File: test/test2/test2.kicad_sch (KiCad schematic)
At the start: 2 parts, among them U1 module_mpu6050, U2 mini_esp32

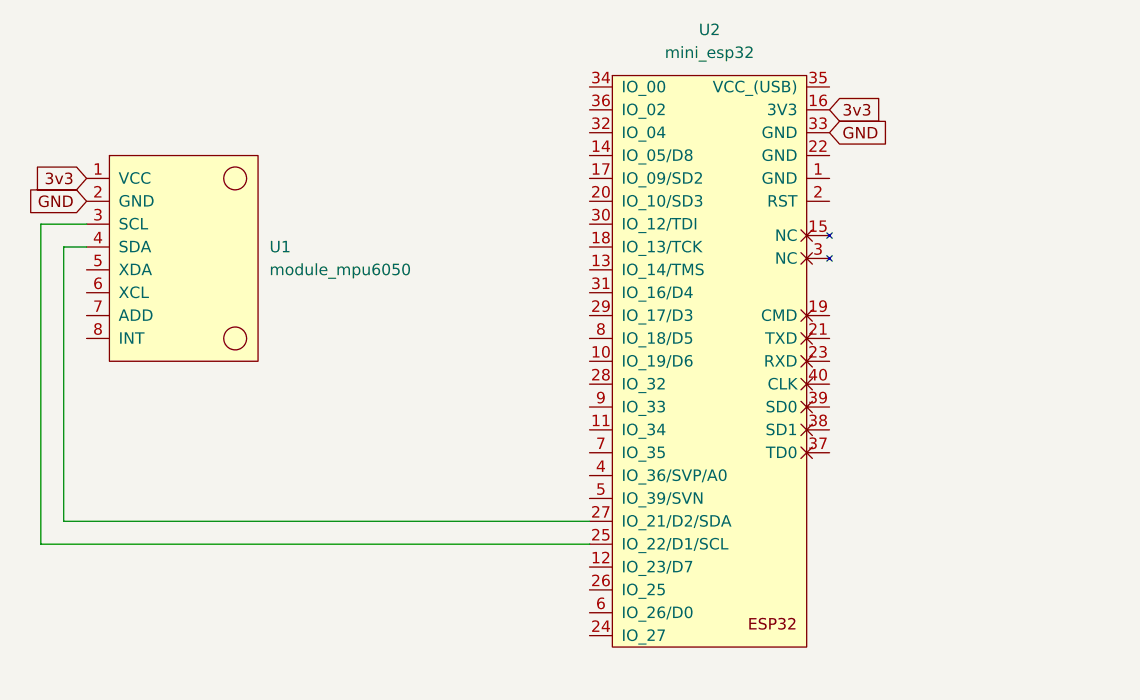
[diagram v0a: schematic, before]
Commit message: update
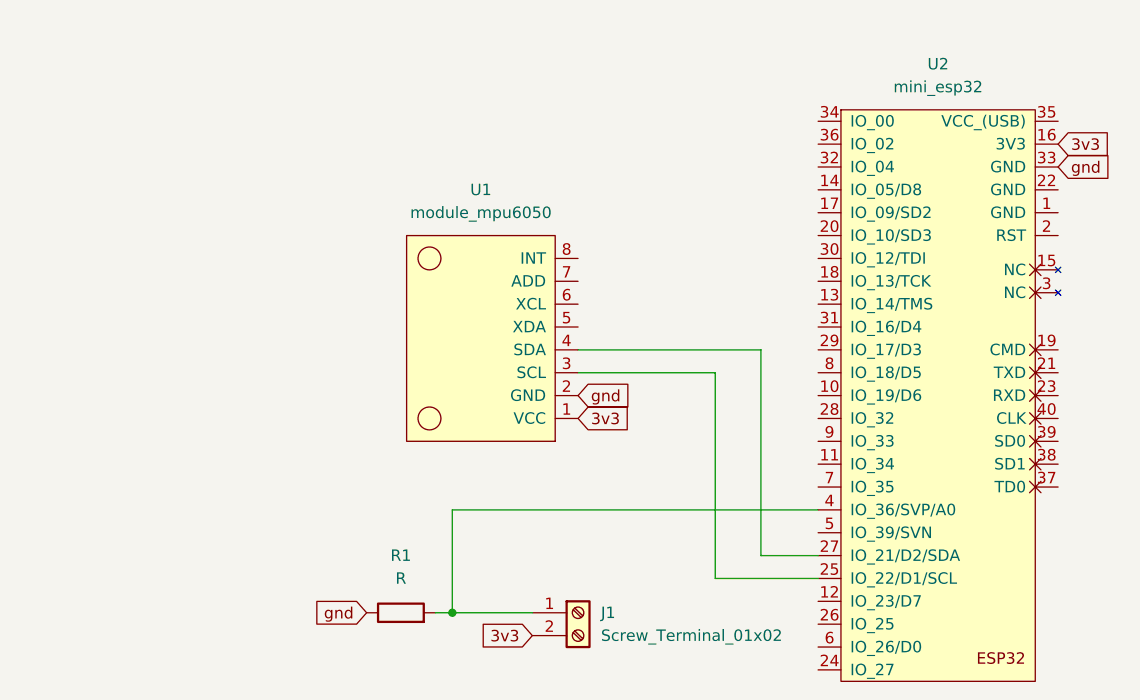
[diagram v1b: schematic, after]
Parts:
- added J1: Screw_Terminal_01x02, Connector_Phoenix_MSTB:PhoenixContact_MSTBA_2,5_2-G-5,08_1x02_P5.08mm_Horizontal, symbol Connector:Screw_Terminal_01x02
- added R1: R, Resistor_THT:R_Axial_DIN0207_L6.3mm_D2.5mm_P10.16mm_Horizontal, symbol Device:R
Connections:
- net 3v3: now also J1.2 (Pin_2)
- net at U2.4 (IO_36/SVP/A0): now also J1.1 (Pin_1), R1.2
- net GND renamed gnd
- net gnd: now also R1.1
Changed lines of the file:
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@@
 (kicad_sch (version 20211123) (generator eeschema)
   (paper "A4")
-  (wire (pts (xy 87.63 55.88) (xy 85.09 55.88))
+  (junction (at 128.27 96.52) (diameter 0) (color 0 0 0 0)
+  )
+  (wire (pts (xy 128.27 96.52) (xy 137.16 96.52))
     (stroke (width 0) (type default) (color 0 0 0 0))
   )
-  (wire (pts (xy 82.55 88.9) (xy 82.55 53.34))
+  (wire (pts (xy 142.24 67.31) (xy 162.56 67.31))
     (stroke (width 0) (type default) (color 0 0 0 0))
   )
-  (wire (pts (xy 85.09 86.36) (xy 143.51 86.36))
+  (wire (pts (xy 157.48 69.85) (xy 157.48 92.71))
     (stroke (width 0) (type default) (color 0 0 0 0))
   )
-  (wire (pts (xy 82.55 53.34) (xy 87.63 53.34))
+  (wire (pts (xy 162.56 90.17) (xy 168.91 90.17))
     (stroke (width 0) (type default) (color 0 0 0 0))
   )
-  (wire (pts (xy 85.09 55.88) (xy 85.09 86.36))
+  (wire (pts (xy 168.91 85.09) (xy 128.27 85.09))
     (stroke (width 0) (type default) (color 0 0 0 0))
   )
-  (wire (pts (xy 143.51 88.9) (xy 82.55 88.9))
+  (wire (pts (xy 162.56 67.31) (xy 162.56 90.17))
     (stroke (width 0) (type default) (color 0 0 0 0))
   )
-  (global_label "3v3" (shape input) (at 87.63 48.26 180) (fields_autoplaced)
+  (wire (pts (xy 157.48 92.71) (xy 168.91 92.71))
+    (stroke (width 0) (type default) (color 0 0 0 0))
+  )
+  (wire (pts (xy 128.27 85.09) (xy 128.27 96.52))
+    (stroke (width 0) (type default) (color 0 0 0 0))
+  )
+  (wire (pts (xy 126.365 96.52) (xy 128.27 96.52))
+    (stroke (width 0) (type default) (color 0 0 0 0))
+  )
+  (wire (pts (xy 142.24 69.85) (xy 157.48 69.85))
+    (stroke (width 0) (type default) (color 0 0 0 0))
+  )
+  (global_label "3v3" (shape input) (at 195.58 44.45 0) (fields_autoplaced)
+    (effects (font (size 1.27 1.27)) (justify left))
+    (property "Intersheet References" "${INTERSHEET_REFS}" (id 0) (at 201.3798 44.3706 0)
+      (effects (font (size 1.27 1.27)) (justify left) hide)
+    )
+  )
+  (global_label "3v3" (shape input) (at 137.16 99.06 180) (fields_autoplaced)
     (effects (font (size 1.27 1.27)) (justify right))
-    (property "Intersheet References" "${INTERSHEET_REFS}" (id 0) (at 81.8302 48.3394 0)
+    (property "Intersheet References" "${INTERSHEET_REFS}" (id 0) (at 131.3602 99.1394 0)
       (effects (font (size 1.27 1.27)) (justify right) hide)
     )
   )
-  (global_label "3v3" (shape input) (at 170.18 40.64 0) (fields_autoplaced)
+  (global_label "3v3" (shape input) (at 142.24 74.93 0) (fields_autoplaced)
     (effects (font (size 1.27 1.27)) (justify left))
-    (property "Intersheet References" "${INTERSHEET_REFS}" (id 0) (at 175.9798 40.5606 0)
+    (property "Intersheet References" "${INTERSHEET_REFS}" (id 0) (at 148.0398 74.8506 0)
       (effects (font (size 1.27 1.27)) (justify left) hide)
     )
   )
-  (global_label "GND" (shape input) (at 170.18 43.18 0) (fields_autoplaced)
+  (global_label "gnd" (shape input) (at 142.24 72.39 0) (fields_autoplaced)
     (effects (font (size 1.27 1.27)) (justify left))
-    (property "Intersheet References" "${INTERSHEET_REFS}" (id 0) (at 176.4636 43.1006 0)
+    (property "Intersheet References" "${INTERSHEET_REFS}" (id 0) (at 148.1002 72.3106 0)
       (effects (font (size 1.27 1.27)) (justify left) hide)
     )
   )
-  (global_label "GND" (shape input) (at 87.63 50.8 180) (fields_autoplaced)
+  (global_label "gnd" (shape input) (at 195.58 46.99 0) (fields_autoplaced)
+    (effects (font (size 1.27 1.27)) (justify left))
+    (property "Intersheet References" "${INTERSHEET_REFS}" (id 0) (at 201.4402 46.9106 0)
+      (effects (font (size 1.27 1.27)) (justify left) hide)
+    )
+  )
+  (global_label "gnd" (shape input) (at 118.745 96.52 180) (fields_autoplaced)
     (effects (font (size 1.27 1.27)) (justify right))
-    (property "Intersheet References" "${INTERSHEET_REFS}" (id 0) (at 81.3464 50.8794 0)
+    (property "Intersheet References" "${INTERSHEET_REFS}" (id 0) (at 112.8848 96.5994 0)
       (effects (font (size 1.27 1.27)) (justify right) hide)
     )
   )
-  (symbol (lib_id "usini_sensors:module_mpu6050") (at 87.63 66.04 0) (unit 1)
+  (symbol (lib_id "ESP32_mini:mini_esp32") (at 181.61 39.37 0) (unit 1)
     (in_bom yes) (on_board yes) (fields_autoplaced)
-    (property "Reference" "U1" (id 0) (at 107.95 55.8799 0)
-      (effects (font (size 1.27 1.27)) (justify left))
-    )
-    (property "Value" "module_mpu6050" (id 1) (at 107.95 58.4199 0)
-      (effects (font (size 1.27 1.27)) (justify left))
-    )
-    (property "Footprint" "usini_sensors:module_mpu6050" (id 2) (at 99.06 72.39 0)
+    (property "Reference" "U2" (id 0) (at 182.245 35.56 0))
+    (property "Value" "mini_esp32" (id 1) (at 182.245 38.1 0))
+    (property "Footprint" "ESP32_mini:ESP32_mini" (id 2) (at 185.42 36.83 0)
       (effects (font (size 1.27 1.27)) hide)
     )
-    (property "Datasheet" "" (id 3) (at 87.63 59.69 0)
-      (effects (font (size 1.27 1.27)) hide)
-    )
-    (pin "1")
-    (pin "2")
-    (pin "3")
-    (pin "4")
-    (pin "5")
-    (pin "6")
-    (pin "7")
-    (pin "8")
-  )
-  (symbol (lib_id "ESP32_mini:mini_esp32") (at 156.21 35.56 0) (unit 1)
-    (in_bom yes) (on_board yes) (fields_autoplaced)
-    (property "Reference" "U2" (id 0) (at 156.845 31.75 0))
-    (property "Value" "mini_esp32" (id 1) (at 156.845 34.29 0))
-    (property "Footprint" "ESP32_mini:ESP32_mini" (id 2) (at 160.02 33.02 0)
-      (effects (font (size 1.27 1.27)) hide)
-    )
-    (property "Datasheet" "" (id 3) (at 160.02 33.02 0)
+    (property "Datasheet" "" (id 3) (at 185.42 36.83 0)
       (effects (font (size 1.27 1.27)) hide)
     )
@@
     (pin "9")
   )
+  (symbol (lib_id "Connector:Screw_Terminal_01x02") (at 142.24 96.52 0) (unit 1)
+    (in_bom yes) (on_board yes) (fields_autoplaced)
+    (property "Reference" "J1" (id 0) (at 144.78 96.5199 0)
+      (effects (font (size 1.27 1.27)) (justify left))
+    )
+    (property "Value" "Screw_Terminal_01x02" (id 1) (at 144.78 99.0599 0)
+      (effects (font (size 1.27 1.27)) (justify left))
+    )
+    (property "Footprint" "Connector_Phoenix_MSTB:PhoenixContact_MSTBA_2,5_2-G-5,08_1x02_P5.08mm_Horizontal" (id 2) (at 142.24 96.52 0)
+      (effects (font (size 1.27 1.27)) hide)
+    )
+    (property "Datasheet" "~" (id 3) (at 142.24 96.52 0)
+      (effects (font (size 1.27 1.27)) hide)
+    )
+    (pin "1")
+    (pin "2")
+  )
+  (symbol (lib_id "Device:R") (at 122.555 96.52 90) (unit 1)
+    (in_bom yes) (on_board yes) (fields_autoplaced)
+    (property "Reference" "R1" (id 0) (at 122.555 90.17 90))
+    (property "Value" "R" (id 1) (at 122.555 92.71 90))
+    (property "Footprint" "Resistor_THT:R_Axial_DIN0207_L6.3mm_D2.5mm_P10.16mm_Horizontal" (id 2) (at 122.555 98.298 90)
+      (effects (font (size 1.27 1.27)) hide)
+    )
+    (property "Datasheet" "~" (id 3) (at 122.555 96.52 0)
+      (effects (font (size 1.27 1.27)) hide)
+    )
+    (pin "1")
+    (pin "2")
+  )
+  (symbol (lib_id "usini_sensors:module_mpu6050") (at 142.24 57.15 180) (unit 1)
+    (in_bom yes) (on_board yes) (fields_autoplaced)
+    (property "Reference" "U1" (id 0) (at 131.445 49.53 0))
+    (property "Value" "module_mpu6050" (id 1) (at 131.445 52.07 0))
+    (property "Footprint" "usini_sensors:module_mpu6050" (id 2) (at 130.81 50.8 0)
+      (effects (font (size 1.27 1.27)) hide)
+    )
+    (property "Datasheet" "" (id 3) (at 142.24 63.5 0)
+      (effects (font (size 1.27 1.27)) hide)
+    )
+    (pin "1")
+    (pin "2")
+    (pin "3")
+    (pin "4")
+    (pin "5")
+    (pin "6")
+    (pin "7")
+    (pin "8")
+  )
   (sheet_instances
     (path "/" (page "1"))
   )
   (symbol_instances
-    (path "/2c91c904-4d5a-4403-a61c-768bb93a8c7e"
+    (path "/6fcbb8e1-110d-45ec-b4b5-1d7e11fb2c45"
+      (reference "J1") (unit 1) (value "Screw_Terminal_01x02") (footprint "Connector_Phoenix_MSTB:PhoenixContact_MSTBA_2,5_2-G-5,08_1x02_P5.08mm_Horizontal")
+    )
+    (path "/8946b347-2cd3-4521-9a24-77ba7a389496"
+      (reference "R1") (unit 1) (value "R") (footprint "Resistor_THT:R_Axial_DIN0207_L6.3mm_D2.5mm_P10.16mm_Horizontal")
+    )
+    (path "/8b16366d-bb35-4e62-87da-7a4d8e7391dd"
       (reference "U1") (unit 1) (value "module_mpu6050") (footprint "usini_sensors:module_mpu6050")
     )
-    (path "/776caef5-77e8-479d-9002-efa59d947083"
+    (path "/58d14422-d631-4dca-8bbe-7d467ce4476e"
       (reference "U2") (unit 1) (value "mini_esp32") (footprint "ESP32_mini:ESP32_mini")
     )
